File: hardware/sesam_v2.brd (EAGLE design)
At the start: 100 x 80 mm, 11 parts, among them X2 C-GRID-06-70543

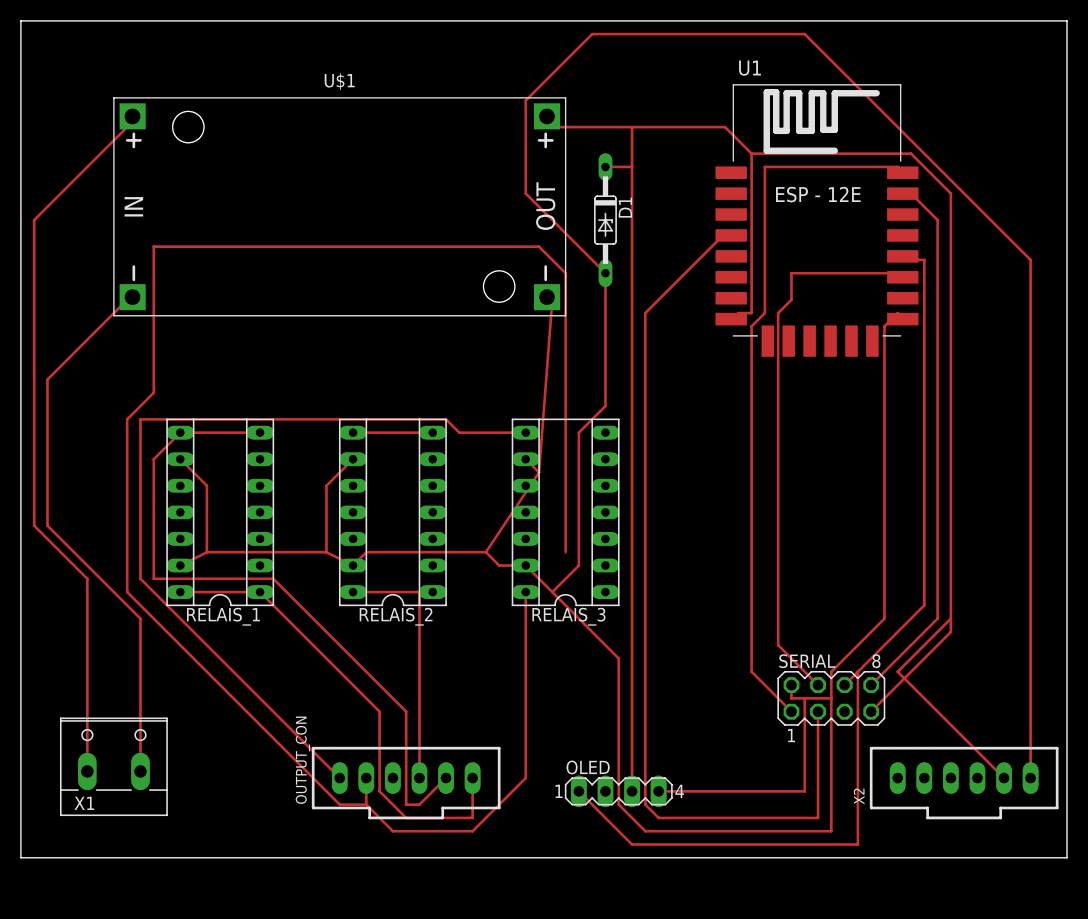
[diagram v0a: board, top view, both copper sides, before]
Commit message: new layout by hallojoh
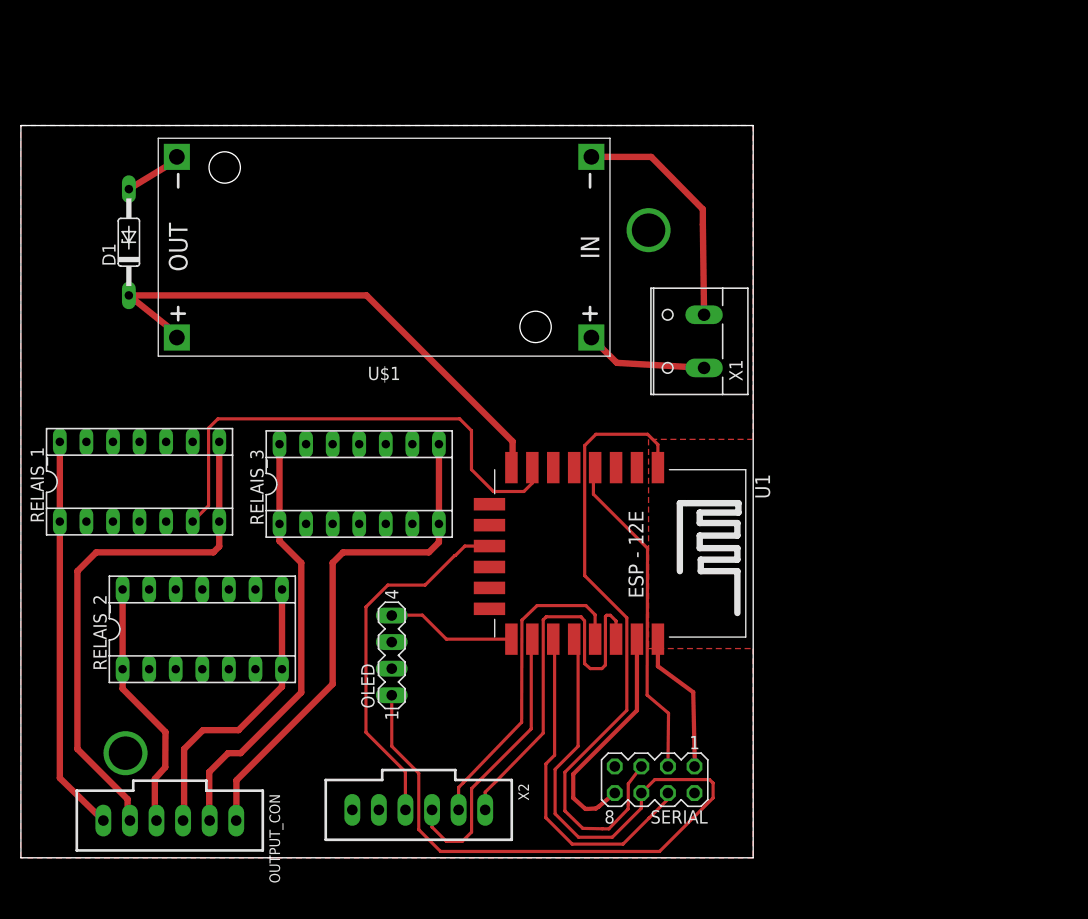
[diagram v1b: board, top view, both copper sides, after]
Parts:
- moved X1 68.9 mm to (64.7, 49.4), turned to 90 degrees
- moved X2 52.2 mm to (38.0, 4.58), turned to 180 degrees
- moved D1 45.6 mm to (10.3, 58.8), turned to 90 degrees
- moved U1 37.2 mm to (55.1, 29.0), turned to 270 degrees
- moved OLED 25.3 mm to (35.5, 19.4), turned to 90 degrees
- moved OUTPUT_CON 23.0 mm to (14.2, 3.56), turned to 180 degrees
- moved RELAIS_2 21.4 mm to (17.3, 21.8), turned to 0 degrees
- moved RELAIS_3 19.9 mm to (32.3, 35.7), turned to 0 degrees
- moved SERIAL 18.6 mm to (60.6, 7.46), turned to 180 degrees
- moved RELAIS_1 8.25 mm to (11.3, 36.0), turned to 0 degrees
- moved U$1 5.73 mm to (34.7, 58.4), turned to 180 degrees
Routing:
- net GND: track 373.0 -> 18.9 mm
- net 3V3: track 199.5 -> 51.9 mm
- net N$7: track 171.2 -> 41.2 mm
- net N$19: track 0.00 -> 61.1 mm
- net N$22: track 68.5 -> 11.8 mm
- net N$18: track 85.6 -> 31.7 mm
- net N$17: track 67.6 -> 13.9 mm
- net N$13: track 0.00 -> 47.7 mm
- net N$9: track 0.00 -> 38.8 mm
- net N$12: track 0.00 -> 35.2 mm
- net N$10: track 0.00 -> 30.8 mm
- net N$8: track 79.5 -> 48.8 mm
- net N$23: track 52.5 -> 22.8 mm
- net N$20: track 51.5 -> 22.6 mm
- net N$11: track 0.00 -> 27.2 mm
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- added copper zone on layer 1, net GND
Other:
- board size 100 x 80 mm -> 70 x 70 mm
